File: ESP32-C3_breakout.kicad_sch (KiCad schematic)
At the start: 26 parts, among them J1 USB4105-GF-A, J2 Conn_01x11_Male, J3 Conn_01x11_Male, SW1 SW_Push, SW2 SW_Push, U1 LD1117S33TR_SOT223, U2 ESP32-C3, U3 WE-TVS-82400102, Y1 40MHz

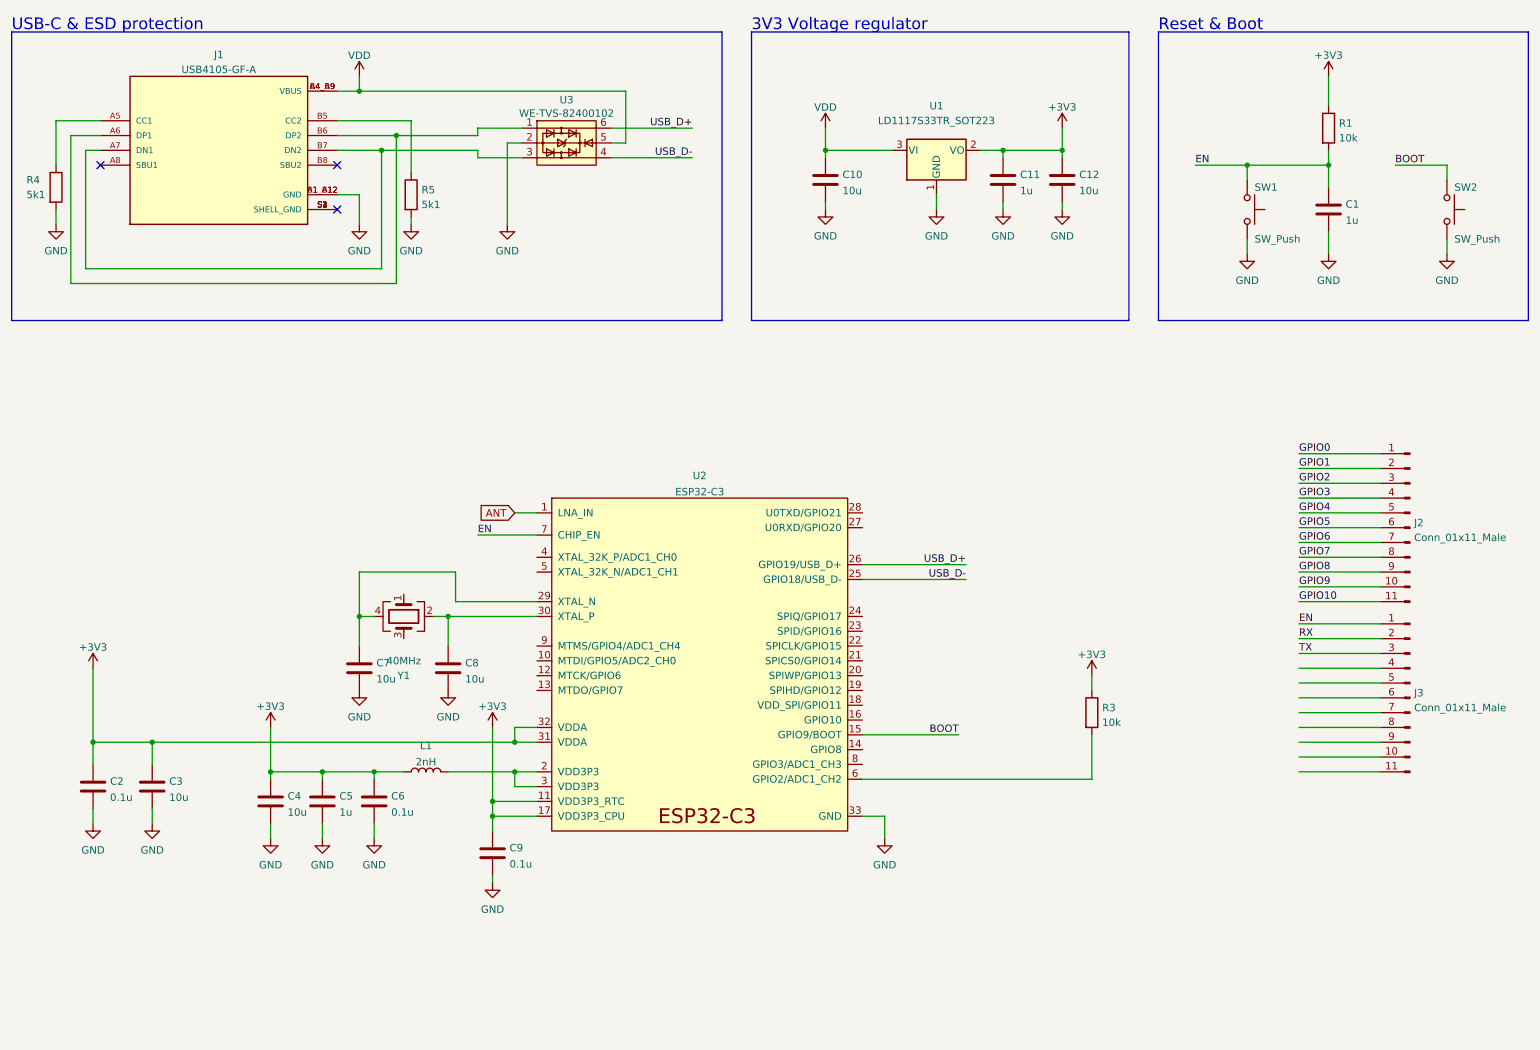
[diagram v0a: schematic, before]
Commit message: Improved schematics
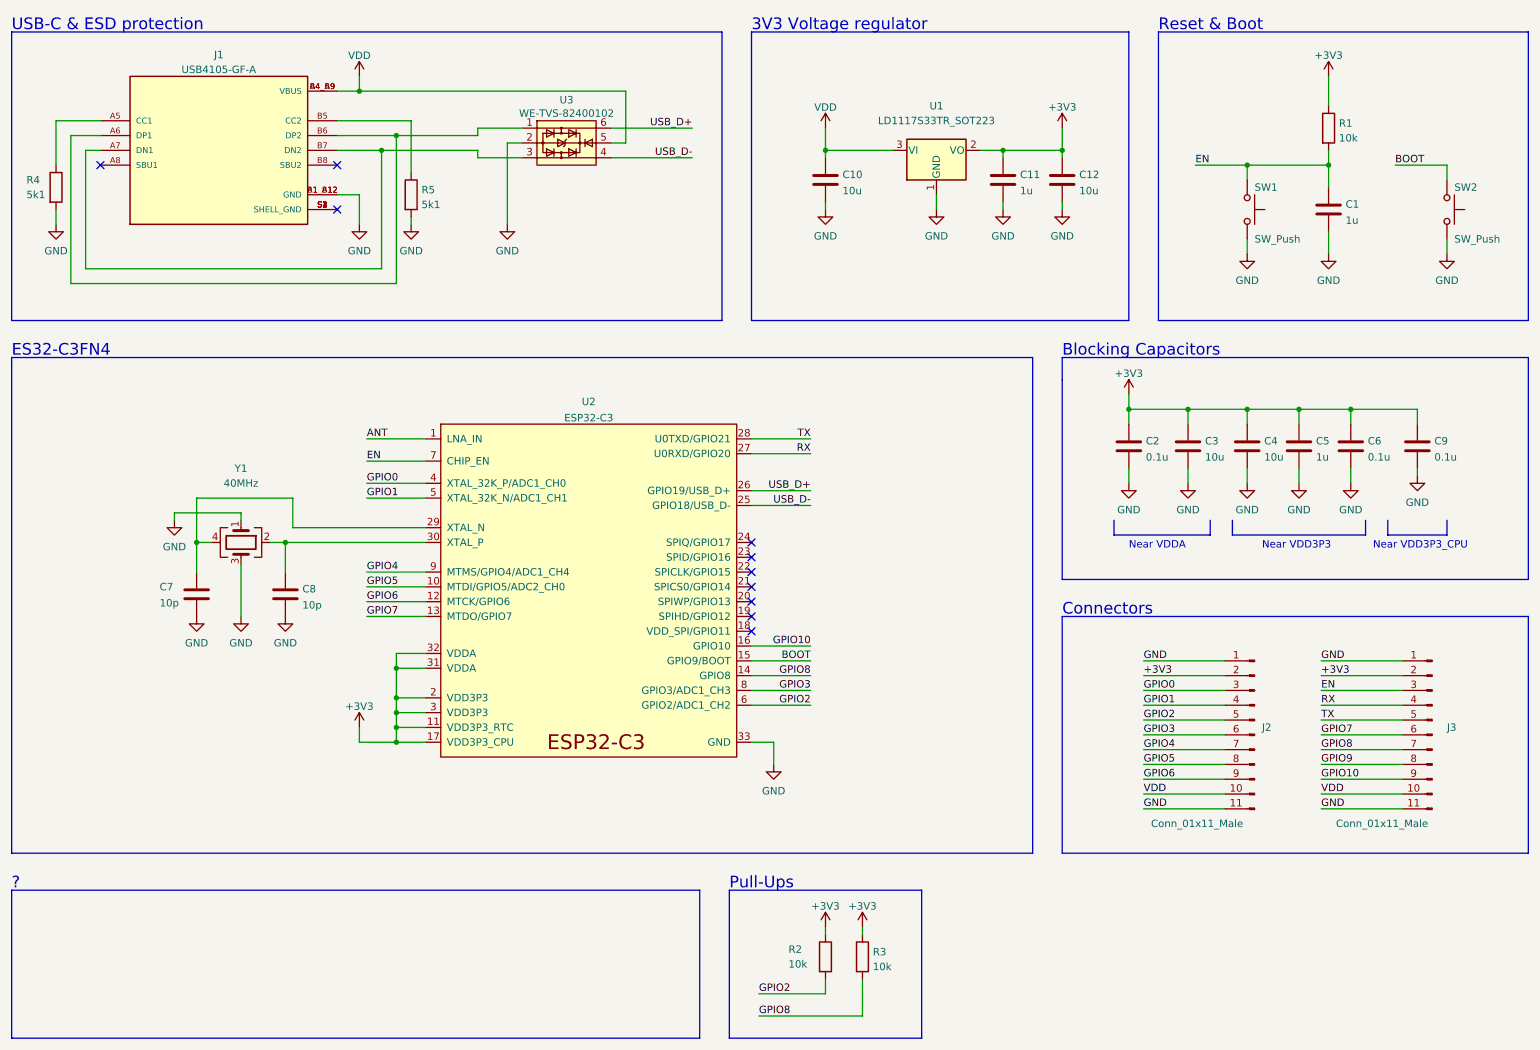
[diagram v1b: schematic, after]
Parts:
- removed L1: 2nH, symbol Device:L
- added R2: 10k, Resistor_SMD:R_0603_1608Metric, symbol Device:R
- C7, C8: value 10u -> 10p
- SW1, SW2: footprint Button_Switch_SMD:SW_SPST_FSMSM -> Button_Switch_SMD:SW_SPST_PTS810
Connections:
- net +3V3: now also J2.2 (Pin_2), J3.2 (Pin_2), U2.2 (VDD3P3), U2.3 (VDD3P3), R2.1
- net EN: now also J3.3 (Pin_3); no longer J3.1 (Pin_1)
- net GND: now also J2.1 (Pin_1), J2.11 (Pin_11), J3.1 (Pin_1), J3.11 (Pin_11), Y1.1, Y1.3
- net GPIO0: now also J2.3 (Pin_3), U2.4 (XTAL_32K_P/ADC1_CH0); no longer J2.1 (Pin_1)
- net GPIO1: now also J2.4 (Pin_4), U2.5 (XTAL_32K_N/ADC1_CH1); no longer J2.2 (Pin_2)
- net GPIO10: now also J3.9 (Pin_9), U2.16 (GPIO10); no longer J2.11 (Pin_11)
- net GPIO2: now also J2.5 (Pin_5), U2.6 (GPIO2/ADC1_CH2), R2.2; no longer J2.3 (Pin_3)
- net GPIO3: now also J2.6 (Pin_6), U2.8 (GPIO3/ADC1_CH3); no longer J2.4 (Pin_4)
- net GPIO4: now also J2.7 (Pin_7), U2.9 (MTMS/GPIO4/ADC1_CH4); no longer J2.5 (Pin_5)
- net GPIO5: now also J2.8 (Pin_8), U2.10 (MTDI/GPIO5/ADC2_CH0); no longer J2.6 (Pin_6)
- net GPIO6: now also J2.9 (Pin_9), U2.12 (MTCK/GPIO6); no longer J2.7 (Pin_7)
- net GPIO7: now also J3.6 (Pin_6), U2.13 (MTDO/GPIO7); no longer J2.8 (Pin_8)
- net GPIO8: now also J3.7 (Pin_7), R3.2, U2.14 (GPIO8); no longer J2.9 (Pin_9)
- net GPIO9: now also J3.8 (Pin_8); no longer J2.10 (Pin_10)
- net RX: now also J3.4 (Pin_4), U2.27 (U0RXD/GPIO20); no longer J3.2 (Pin_2)
- net TX: now also J3.5 (Pin_5), U2.28 (U0TXD/GPIO21); no longer J3.3 (Pin_3)
- net VDD: now also J2.10 (Pin_10), J3.10 (Pin_10)
- no-connect marks 3 -> 10
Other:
- note added: "?"
- note added: "Blocking Capacitors"
- note added: "Connectors"
- note added: "ES32-C3FN4"
- note added: "Near VDD3P3"
- note added: "Near VDD3P3_CPU"
- note added: "Near VDDA"
- note added: "Pull-Ups"
- title: (none) -> ESP32-C3 Nano
- moved on the sheet: C2, C3, C4, C5, C6, C7, C8, C9, J2, J3, R3, U2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
